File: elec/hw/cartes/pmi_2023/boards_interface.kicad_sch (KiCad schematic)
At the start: 2 parts

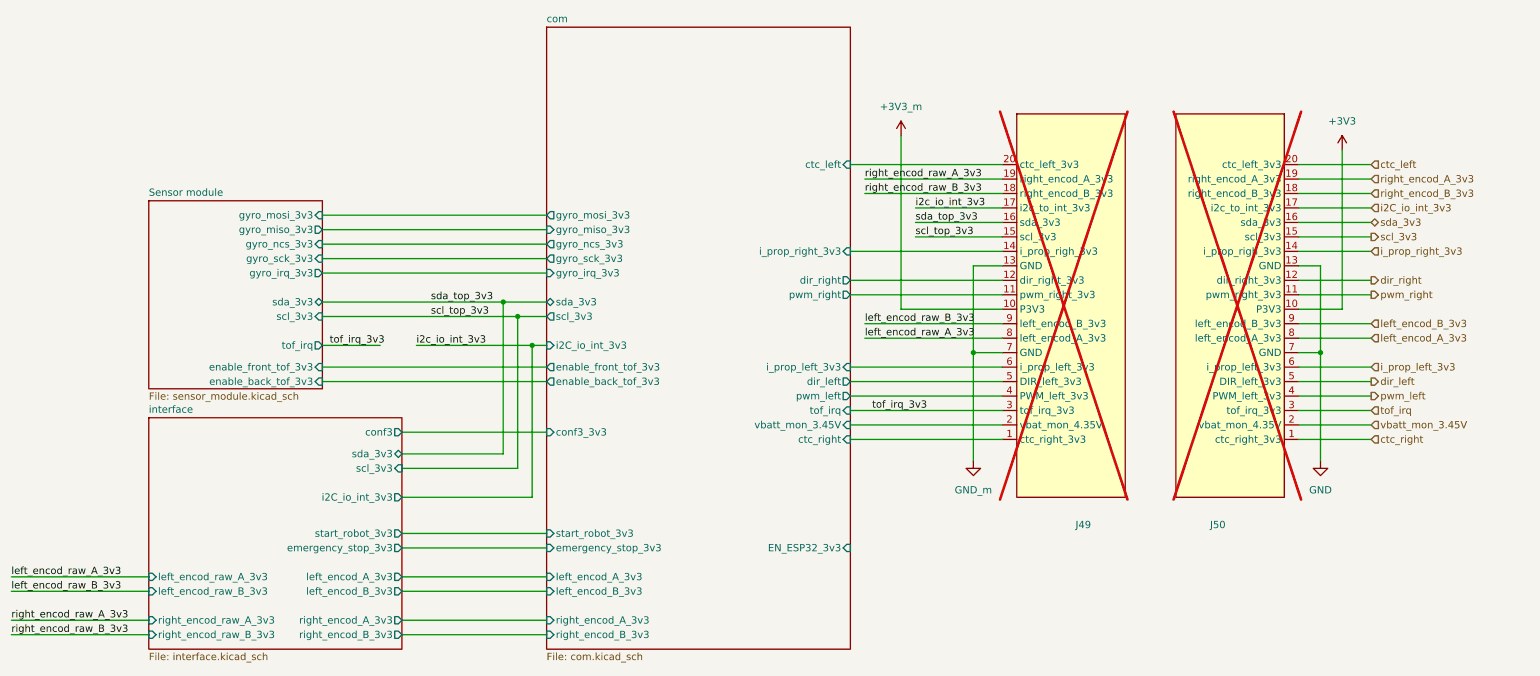
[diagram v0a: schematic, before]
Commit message: pmi board V2, ready for review
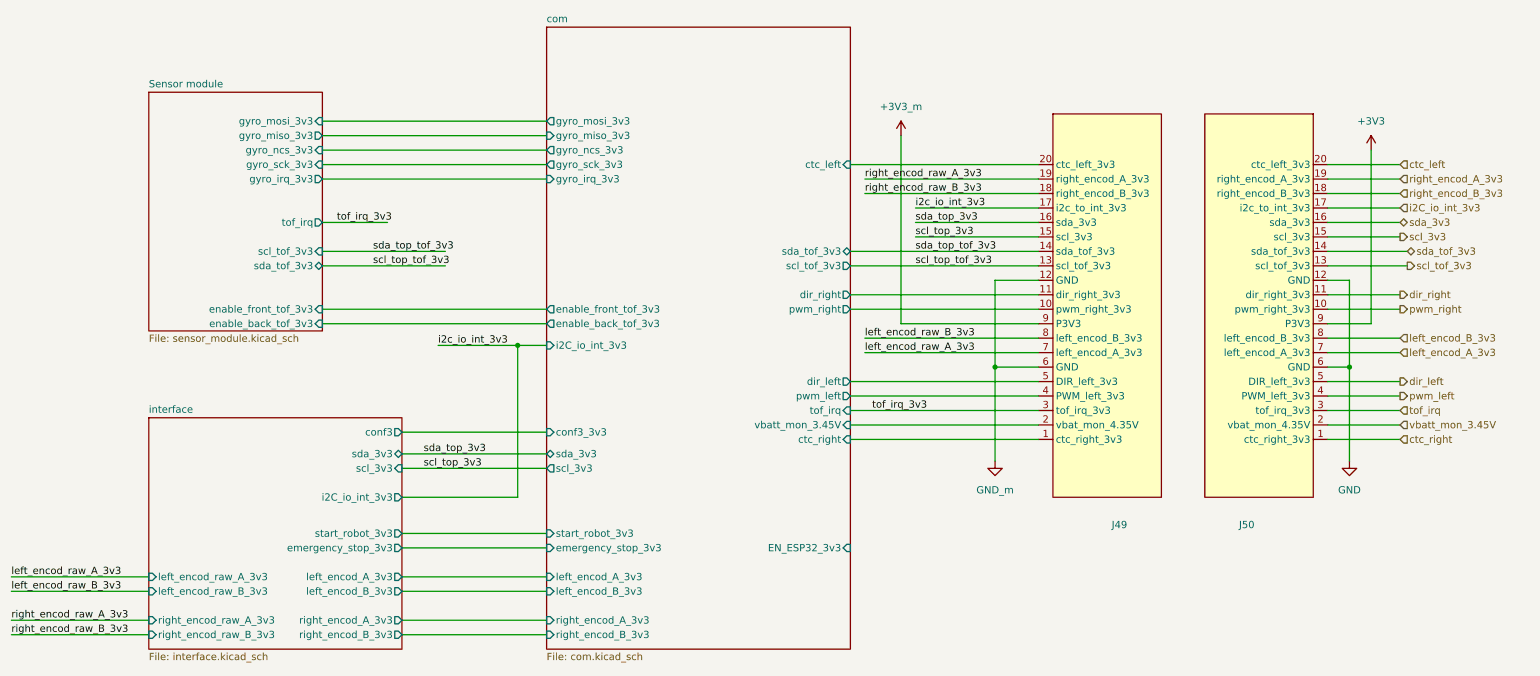
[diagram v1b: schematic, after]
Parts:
- J49: footprint pmi_2023_specific:pmi_2023_interconnection_top -> pmi_2023_specific:pmi_2023_interconnection; symbol pmi_2023_specific:interconnect -> pmi_2023_specific:interconnect_V2; now fitted
- J50: symbol pmi_2023_specific:interconnect -> pmi_2023_specific:interconnect_V2; now fitted
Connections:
- net com/i_prop_left_3v3 is gone; now on net GND_m: J49.6 (GND)
- net i_prop_left_3v3 is gone; now on net GND: J50.6 (GND)
- net +3V3: now also J50.9 (P3V3); no longer J50.10 (P3V3)
- net +3V3_m: now also J49.9 (P3V3); no longer J49.10 (P3V3)
- net GND: now also J50.12 (GND); no longer J50.13 (GND), J50.7 (GND)
- net GND_m: now also J49.12 (GND); no longer J49.13 (GND), J49.7 (GND)
- net com/dir_right: now also J49.11 (dir_right_3v3); no longer J49.12 (dir_right_3v3)
- net com/pwm_right: now also J49.10 (pwm_right_3v3); no longer J49.11 (pwm_right_3v3)
- net dir_right: now also J50.11 (dir_right_3v3); no longer J50.12 (dir_right_3v3)
- net left_encod_A_3v3: now also J50.7 (left_encod_A_3v3); no longer J50.8 (left_encod_A_3v3)
- net left_encod_B_3v3: now also J50.8 (left_encod_B_3v3); no longer J50.9 (left_encod_B_3v3)
- net left_encod_raw_A_3v3: now also J49.7 (left_encod_A_3v3); no longer J49.8 (left_encod_A_3v3)
- net left_encod_raw_B_3v3: now also J49.8 (left_encod_B_3v3); no longer J49.9 (left_encod_B_3v3)
- net pwm_right: now also J50.10 (pwm_right_3v3); no longer J50.11 (pwm_right_3v3)
- net com/i_prop_right_3v3 renamed sda_top_tof_3v3
- net i_prop_right_3v3 renamed sda_tof_3v3
- new net scl_tof_3v3: J50.13 (scl_tof_3v3)
- new net scl_top_tof_3v3: J49.13 (scl_tof_3v3)
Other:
- sheet Sensor module ports: added scl_tof_3v3, sda_tof_3v3; removed scl_3v3, sda_3v3
- sheet com ports: added scl_tof_3v3, sda_tof_3v3; removed i_prop_left_3v3, i_prop_right_3v3

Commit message: pmi board V2, ready for review
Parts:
- J50: footprint pmi_2023_specific:pmi_2023_interconnection -> pmi_2023_specific:pmi_2023_interconnection_bot
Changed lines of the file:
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@@
 			)
 		)
-		(property "Footprint" "pmi_2023_specific:pmi_2023_interconnection"
+		(property "Footprint" "pmi_2023_specific:pmi_2023_interconnection_bot"
 			(at 242.57 93.98 0)
 			(effects
